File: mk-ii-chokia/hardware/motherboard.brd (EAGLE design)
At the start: 100 x 165.1 mm, 26 parts, among them SW1 CHERRY_MX, SW10 CHERRY_MX, SW11 CHERRY_MX, SW12 CHERRY_MX, SW13 CHERRY_MX, SW14 CHERRY_MX, SW15 CHERRY_MX, SW2 CHERRY_MX, SW3 CHERRY_MX, SW4 CHERRY_MX, SW5 CHERRY_MX, SW6 CHERRY_MX, SW7 CHERRY_MX, SW8 CHERRY_MX, SW9 CHERRY_MX, T2 BC337

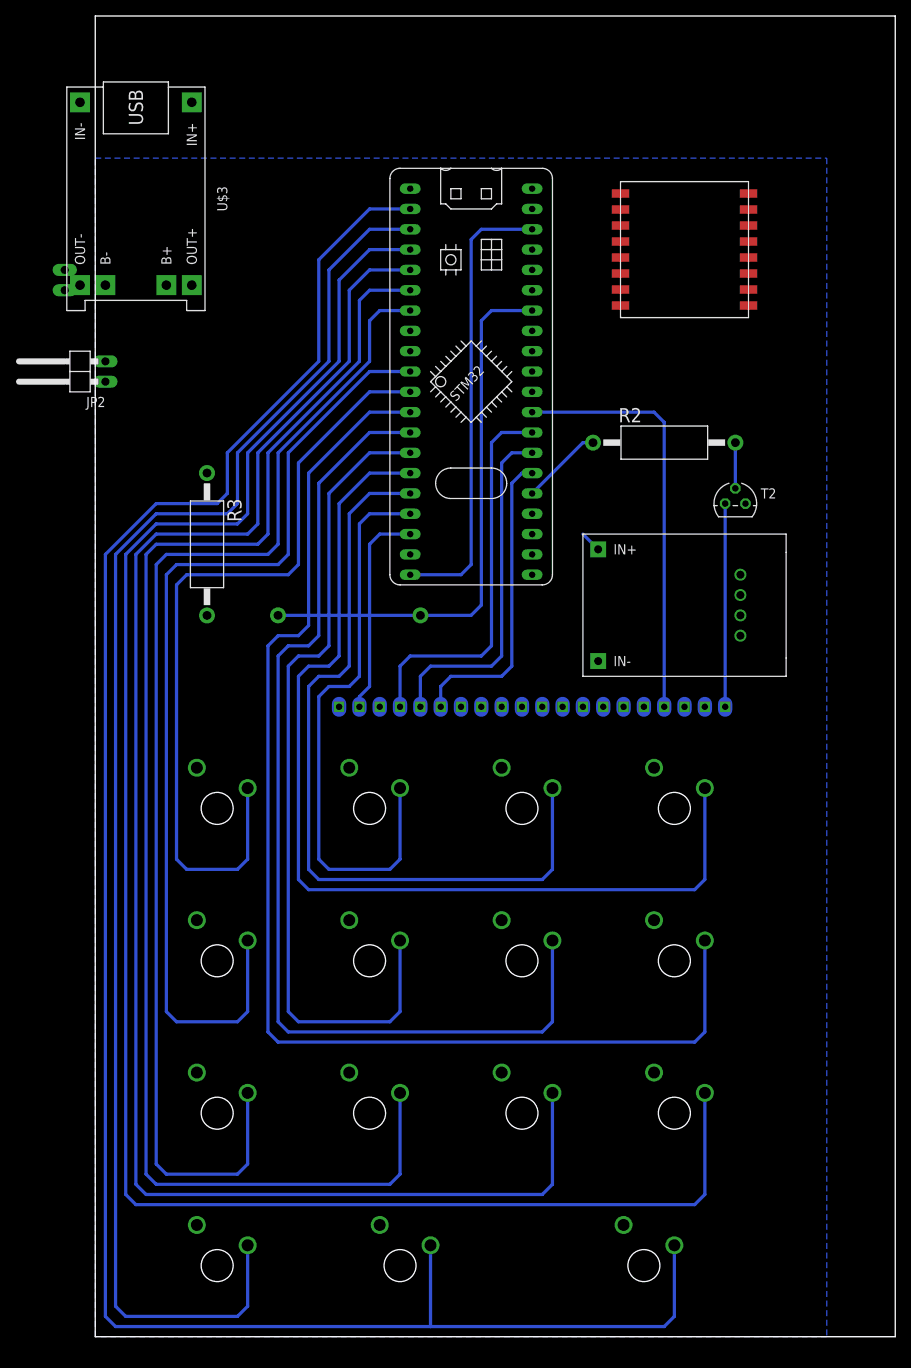
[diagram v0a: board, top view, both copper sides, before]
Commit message: Ready 2 etch dot com?
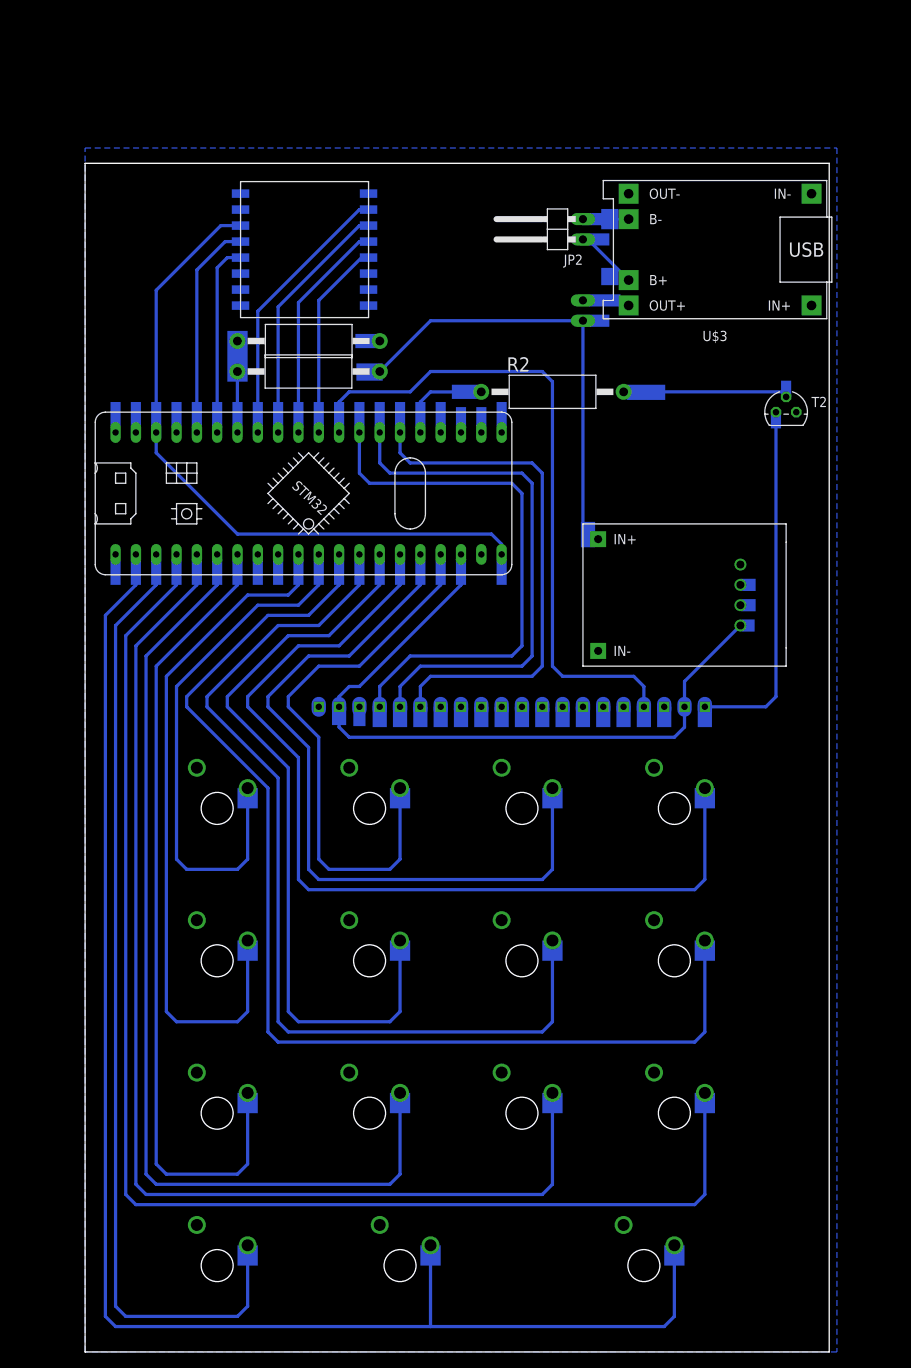
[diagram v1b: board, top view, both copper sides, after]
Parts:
- moved U$3 72.7 mm to (77.5, 135.9), turned to 180 degrees
- moved JP1 64.9 mm to (57.1, 128.3)
- moved JP2 62.3 mm to (57.1, 138.4)
- moved U$4 47.5 mm to (26.2, 135.9)
- moved U$2 37.1 mm to (17.8, 105.4), turned to 90 degrees
- moved R7 34.7 mm to (26.7, 124.5), flipped to the top, turned to 0 degrees
- moved R3 25.0 mm to (26.7, 120.7), turned to 180 degrees
- moved R2 15.3 mm to (57.1, 118.1)
- moved T2 13.1 mm to (86.4, 115.6)
- moved U$1 2.54 mm to (43.2, 111.8)
- moved U$5 1.27 mm to (73.7, 92.7)
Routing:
- net N$29: track 252.9 -> 188.1 mm
- net +5V: track 26.5 -> 88.5 mm
- net N$28: track 183.2 -> 121.3 mm
- net N$31: track 227.9 -> 168.8 mm
- net N$24: track 68.4 -> 11.4 mm
- net N$30: track 202.7 -> 146.4 mm
- net N$27: track 177.5 -> 124.1 mm
- net N$16: track 2.69 -> 56.1 mm
- net N$26: track 150.9 -> 101.8 mm
- net N$25: track 123.2 -> 87.1 mm
- net N$4: track 0.00 -> 34.3 mm
- net N$23: track 99.8 -> 67.3 mm
- net N$5: track 0.00 -> 31.2 mm
- net N$11: track 52.6 -> 83.2 mm
- net N$6: track 0.00 -> 28.2 mm
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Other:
- board size 100 x 165.1 mm -> 93 x 148.6 mm
